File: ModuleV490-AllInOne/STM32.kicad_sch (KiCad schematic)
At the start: 46 parts, among them J1 SPI_DEBUG, J10 TEMP2, J11 TEMP1, J12 TEMP2, J13 TEMP3, J2 BOOT_MODE, J3 UART_PROG, J4 ST_LINK, J8 TXRX, Q1 AO3401A, U13 EL3H7(B)(TA)-G, U4 RELAY1, U5 STM32F030K6Tx, Y1 8MHZ

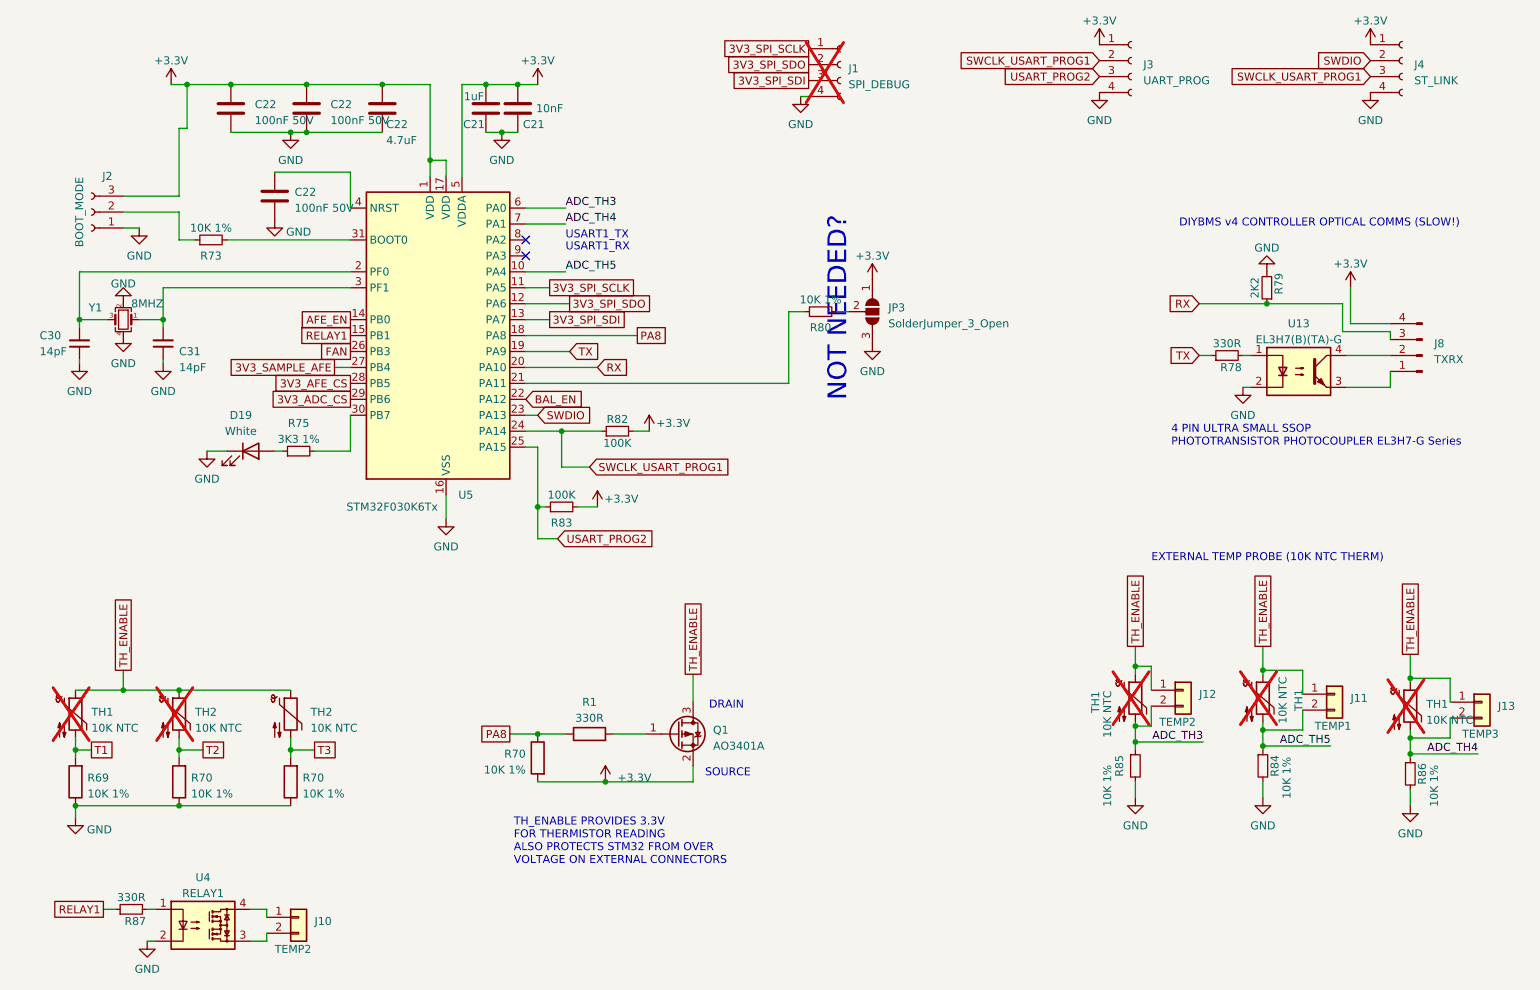
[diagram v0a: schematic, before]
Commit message: Squashed commit of the following:
commit 382df4b7a104fb34cc4a4da3f786b21ade19fcd5
Author: GitHub Action <action@github.com>
Date:   Fri Apr 18 11:47:05 2025 +0000

    CI: pcb-artifacts-ModuleV490-AllInOne

commit b35cb7a0d3894cf57b33edb037eb829bc9ec5ea4
Author: Stuart Pittaway <1201909+stuartpittaway@users.noreply.github.com>
Date:   Fri Apr 18 12:44:57 2025 +0100

    Minor tweaks

commit ea046b7e5d836263693da1b47c6dfb3dc918925c
Author: Stuart Pittaway <1201909+stuartpittaway@users.noreply.github.com>
Date:   Fri Apr 18 12:44:16 2025 +0100

    PCB Panel of Temp sensors

commit ba929f4700586b6858203bc466c6b18e911d661e
Author: GitHub Action <action@github.com>
Date:   Sun Mar 23 15:29:50 2025 +0000

    CI: pcb-artifacts-ModuleV490-AllInOne

commit 1dbbac7378fdc5acb48c43d3f728917ce2318f16
Author: GitHub Action <action@github.com>
Date:   Wed Apr 10 09:57:21 2024 +0000

    CI: pcb-artifacts-ModuleV490-AllInOne

commit 35f617d42fc7a6a7ab395d232005d3307c26595c
Author: Stuart Pittaway <1201909+stuartpittaway@users.noreply.github.com>
Date:   Wed Apr 10 10:55:49 2024 +0100

    Update pcb-artifacts-modulev490-allinone.yaml

commit c8295c0089ea2c5e86742be6a5572142963deb8f
Author: Stuart Pittaway <1201909+stuartpittaway@users.noreply.github.com>
Date:   Wed Apr 10 10:53:50 2024 +0100

    Update pcb-artifacts-modulev490-allinone.yaml

commit d19b2989a6afd4cac4ecf3c8c78554eedba7b99a
Author: Stuart Pittaway <1201909+stuartpittaway@users.noreply.github.com>
Date:   Wed Apr 10 10:50:28 2024 +0100

    Update pcb-artifacts-modulev490-allinone.yaml

commit 8478886fe70d1ee53aca3bbd908099e6f38ff11d
Author: Stuart Pittaway <1201909+stuartpittaway@users.noreply.github.com>
Date:   Wed Apr 10 10:41:28 2024 +0100

    Update pcb-artifacts-modulev490-allinone.yaml

commit afeafa74721a9b51459c6106f0a15ae423229204
Author: Stuart Pittaway <1201909+stuartpittaway@users.noreply.github.com>
Date:   Wed Apr 10 10:39:10 2024 +0100

    Inductor part change - fix workflows

commit 70fd25ba43b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
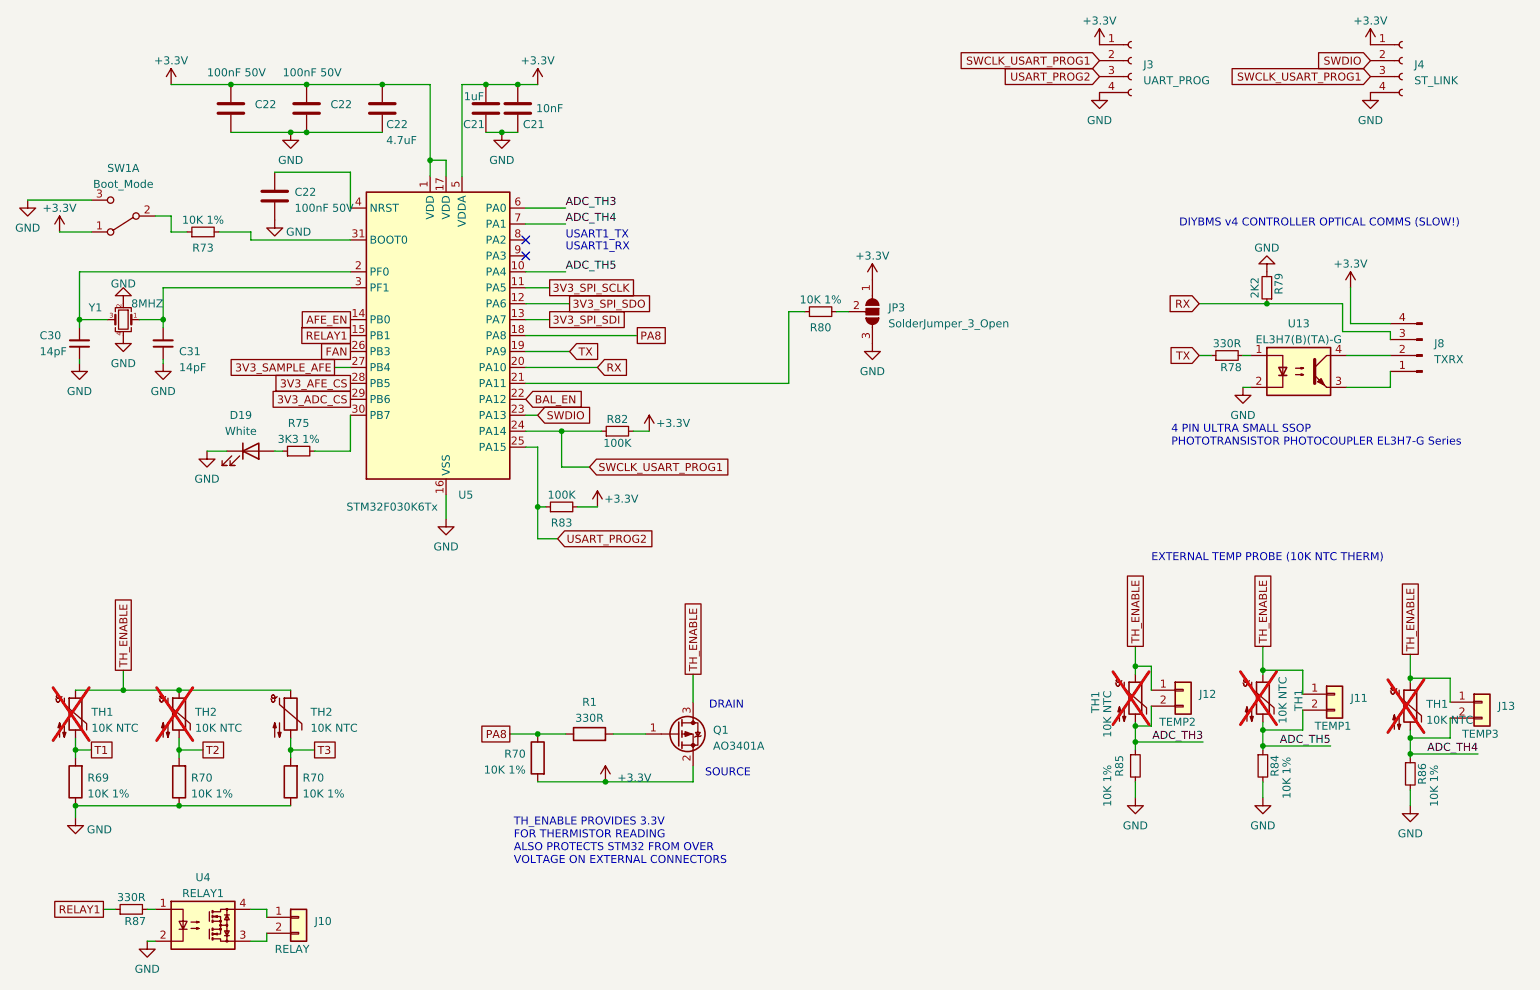
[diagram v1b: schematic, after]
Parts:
- removed J1: SPI_DEBUG, Connector_PinSocket_2.00mm:PinSocket_1x04_P2.00mm_Vertical, symbol Connector:Conn_01x04_Socket
- removed J2: BOOT_MODE, Connector_PinHeader_2.54mm:PinHeader_1x03_P2.54mm_Vertical, symbol Connector:Conn_01x03_Socket
- added SW1: Boot_Mode, SHOU_HAN:MST22D18G2 125, symbol Switch:SW_DPDT_x2
- C30, C31: footprint Capacitor_SMD:C_0805_2012Metric -> Capacitor_SMD:C_0402_1005Metric; LCSCStockCode C519919 -> C458857; PartNumber CC0805JRNPO9BN140 -> 0402N140J500CT
- J10: value TEMP2 -> RELAY; footprint Connector_JST:JST_PH_S2B-PH-K_1x02_P2.00mm_Horizontal -> Connector_JST:JST_PH_S2B-PH-SM4-TB_1x02-1MP_P2.00mm_Horizontal; LCSCStockCode C265016 -> C295747; PartNumber S2B-PH-K(LF)(SN) -> S2B-PH-SM4-TB(LF)(SN)
- J11, J12, J13: footprint Connector_JST:JST_PH_S2B-PH-K_1x02_P2.00mm_Horizontal -> Connector_JST:JST_PH_S2B-PH-SM4-TB_1x02-1MP_P2.00mm_Horizontal; LCSCStockCode C265016 -> C295747; PartNumber S2B-PH-K(LF)(SN) -> S2B-PH-SM4-TB(LF)(SN)
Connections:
- net +3.3V: now also SW1.1 (A)
- net GND: now also SW1.3 (C)
- net at R73.1: now also SW1.2 (B)
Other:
- note removed: "NOT NEEDED?"
- moved on the sheet: R73
